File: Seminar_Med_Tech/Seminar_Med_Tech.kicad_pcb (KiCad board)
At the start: 2 copper layers, 96 x 88 mm, 167 parts, among them J1 CONN_02X08, J3 CONN_02X10, J5 CONN_02X10, J6 DB15_F-RA, J7 CONN_02X08, U1 OPA132, U18 ADS1298, U20 ADS1298, U4 LM317T, U5 LM317T, U6 LM337K

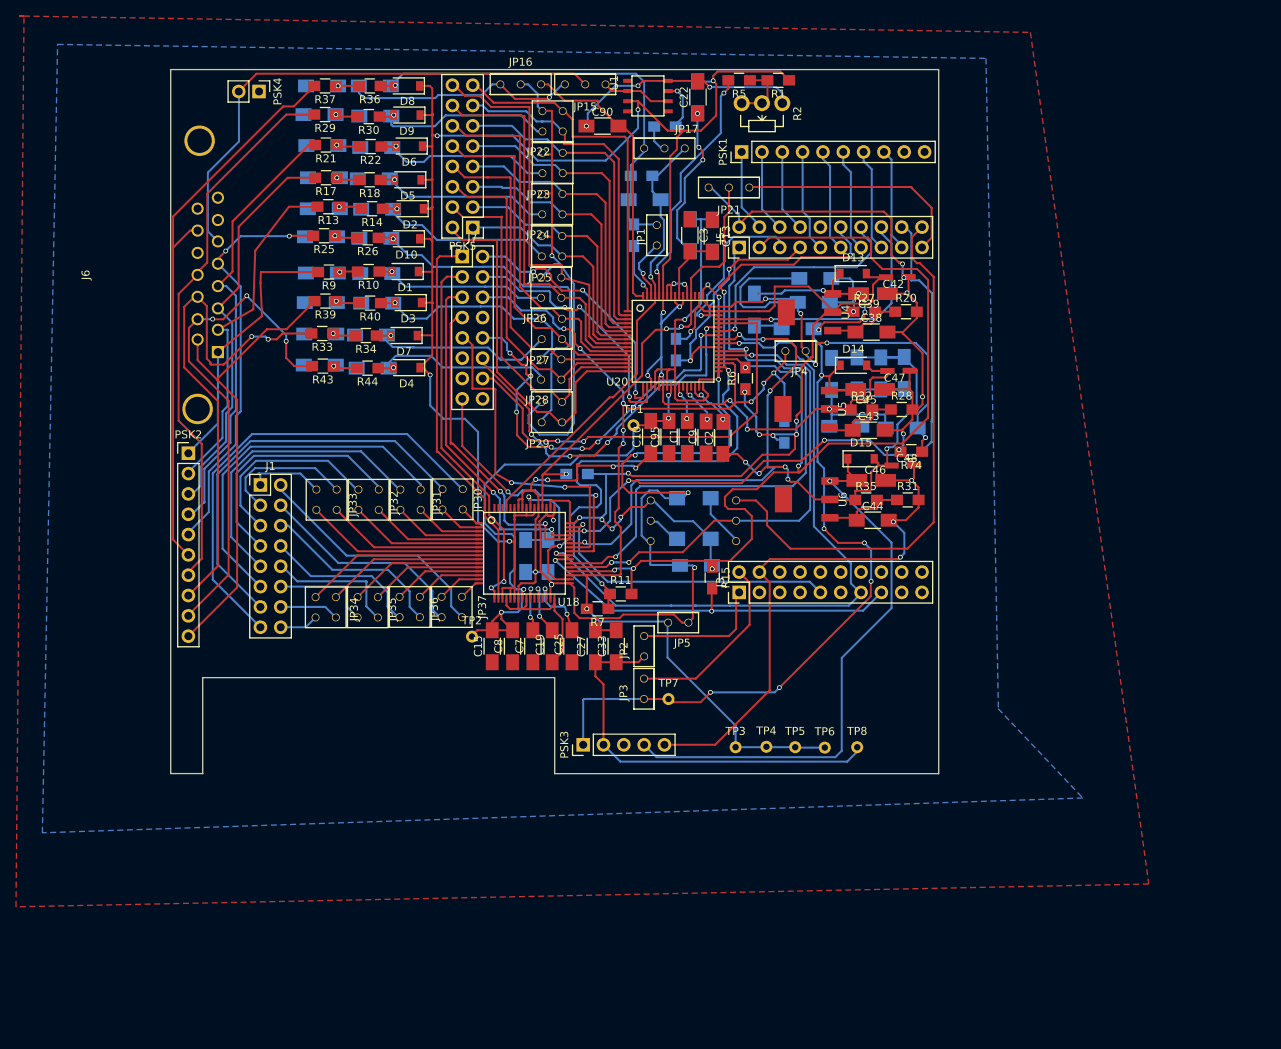
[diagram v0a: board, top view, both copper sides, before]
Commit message: Update
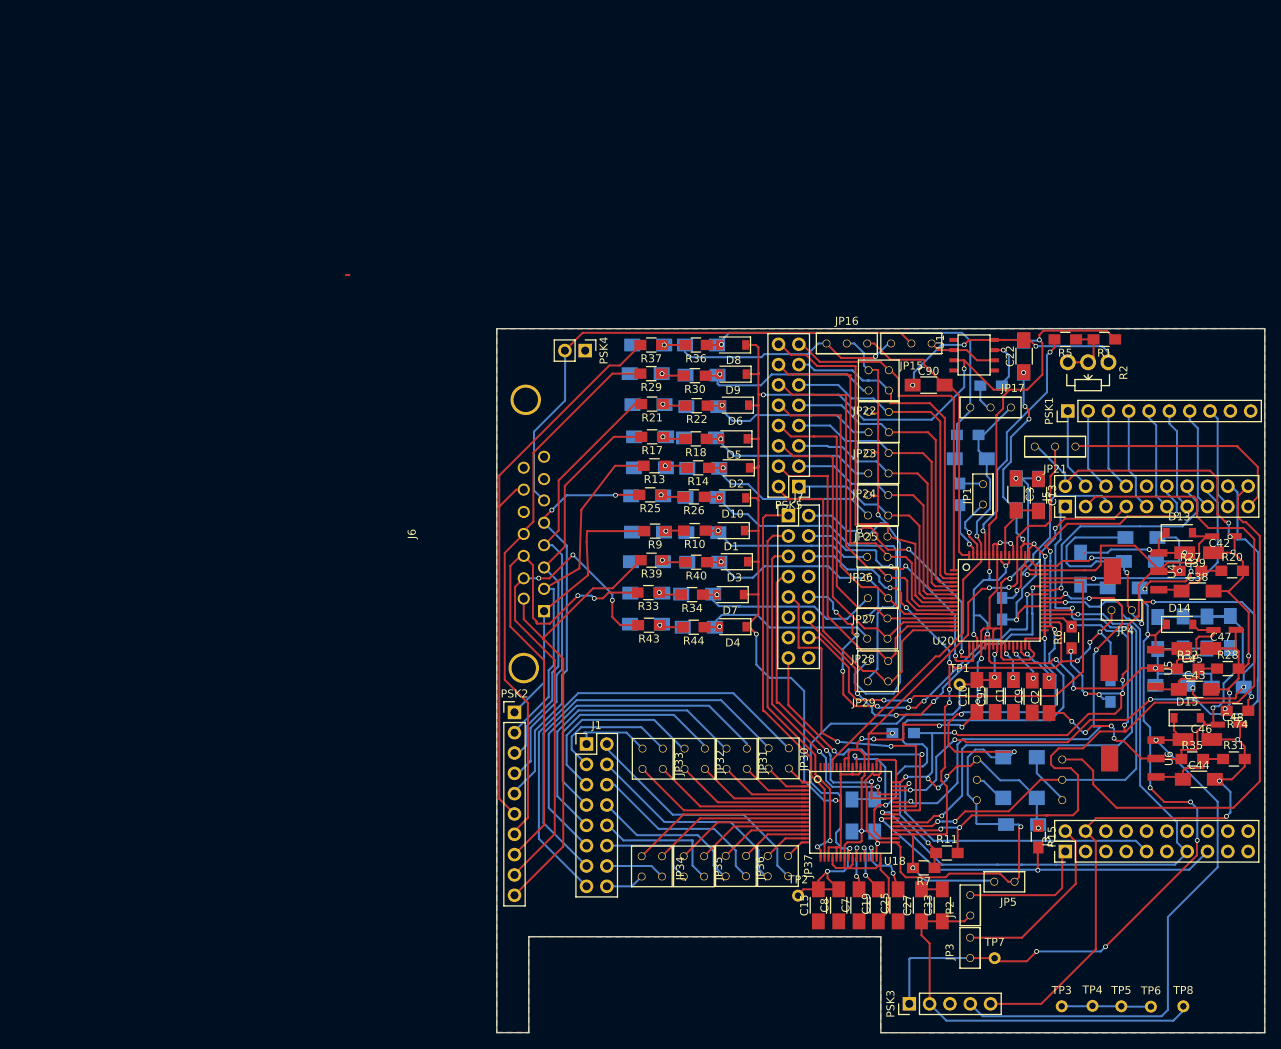
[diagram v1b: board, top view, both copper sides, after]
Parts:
- moved C35 52.2 mm to (139.4, 115.8)
- moved C34 52.1 mm to (136.6, 115.8)
- moved TP6 52.1 mm to (174.0, 139.7)
- moved C42 52.1 mm to (182.5, 81.3)
- moved C48 52.1 mm to (184.2, 104.1)
- moved R32 52.1 mm to (178.6, 97.5)
- moved C15 52.1 mm to (132.4, 127.1)
- moved C22 52.1 mm to (158.1, 58.4)
- moved C23 52.1 mm to (117.4, 92.3)
- moved C24 52.1 mm to (110.8, 91.9)
- moved C27 52.1 mm to (145.3, 127.1)
- moved C33 52.1 mm to (147.9, 127.1)
- moved C74 52.1 mm to (118.0, 84.2)
- moved C80 52.1 mm to (111.3, 72.4)
- moved D2 52.1 mm to (122.1, 72.4)
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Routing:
- net AVSS: track 195.5 -> 214.7 mm, vias 16 -> 20
- net /PWDN: track 111.2 -> 106.8 mm
- net /RESET: track 131.0 -> 132.8 mm
- net AVDD: track 272.1 -> 273.9 mm
- net AGND: track 262.7 -> 264.3 mm, vias 18 -> 20

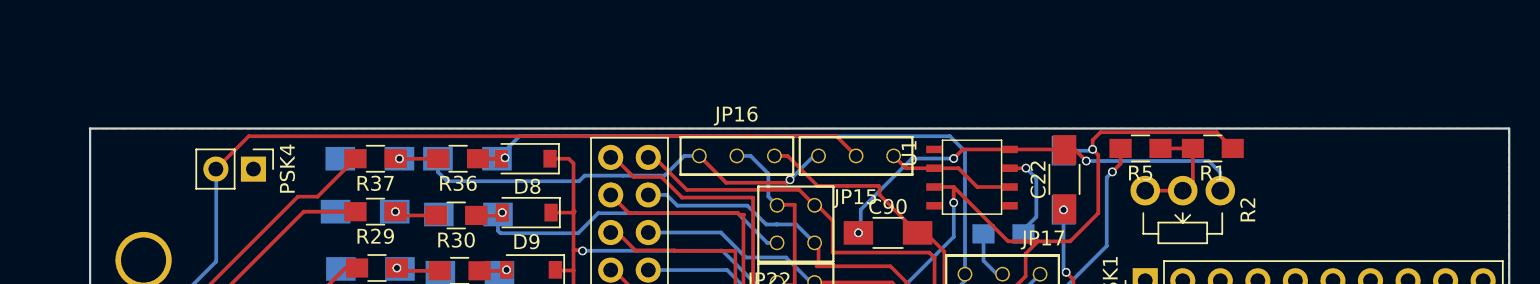
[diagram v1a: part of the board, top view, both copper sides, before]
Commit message: Update
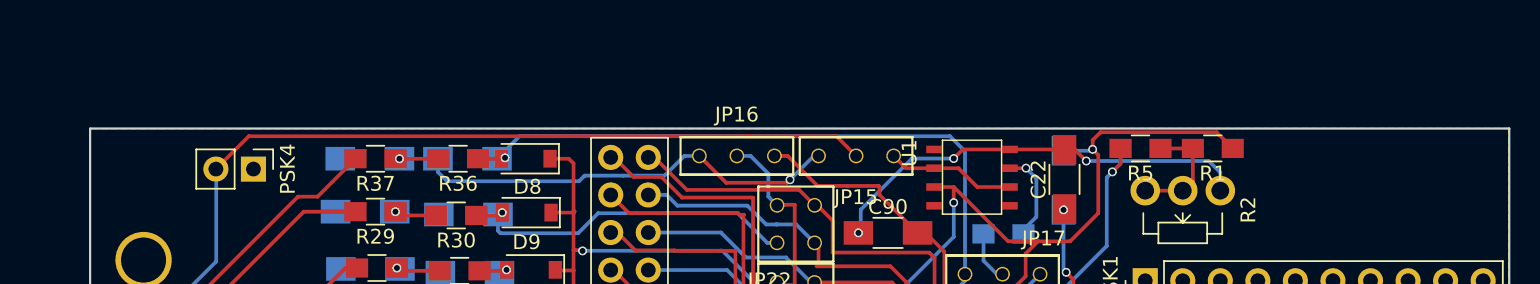
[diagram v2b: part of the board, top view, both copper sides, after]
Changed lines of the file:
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@@
     (links 422)
     (no_connects 0)
-    (area 32.1 15.9 173.700001 127.250001)
+    (area 92.126999 54.903299 188.281301 143.066001)
     (thickness 1.6)
     (drawings 8)
@@
   (gr_line (start 188.202 142.991) (end 140.202 142.991) (angle 90) (layer Edge.Cuts) (width 0.15))
   (gr_line (start 188.202 54.991) (end 188.202 142.991) (angle 90) (layer Edge.Cuts) (width 0.15))
-  (gr_line (start 92.1809 54.9783) (end 188.1809 54.9783) (angle 90) (layer Edge.Cuts) (width 0.15))
+  (gr_line (start 92.2063 54.9783) (end 188.2063 54.9783) (angle 90) (layer Edge.Cuts) (width 0.15))
   (segment (start 165.6715 82.9945) (end 165.7004 82.9656) (width 0.25) (layer F.Cu) (net 0))
   (segment (start 155.7535 94.615) (end 155.7535 95.492) (width 0.25) (layer F.Cu) (net 1))

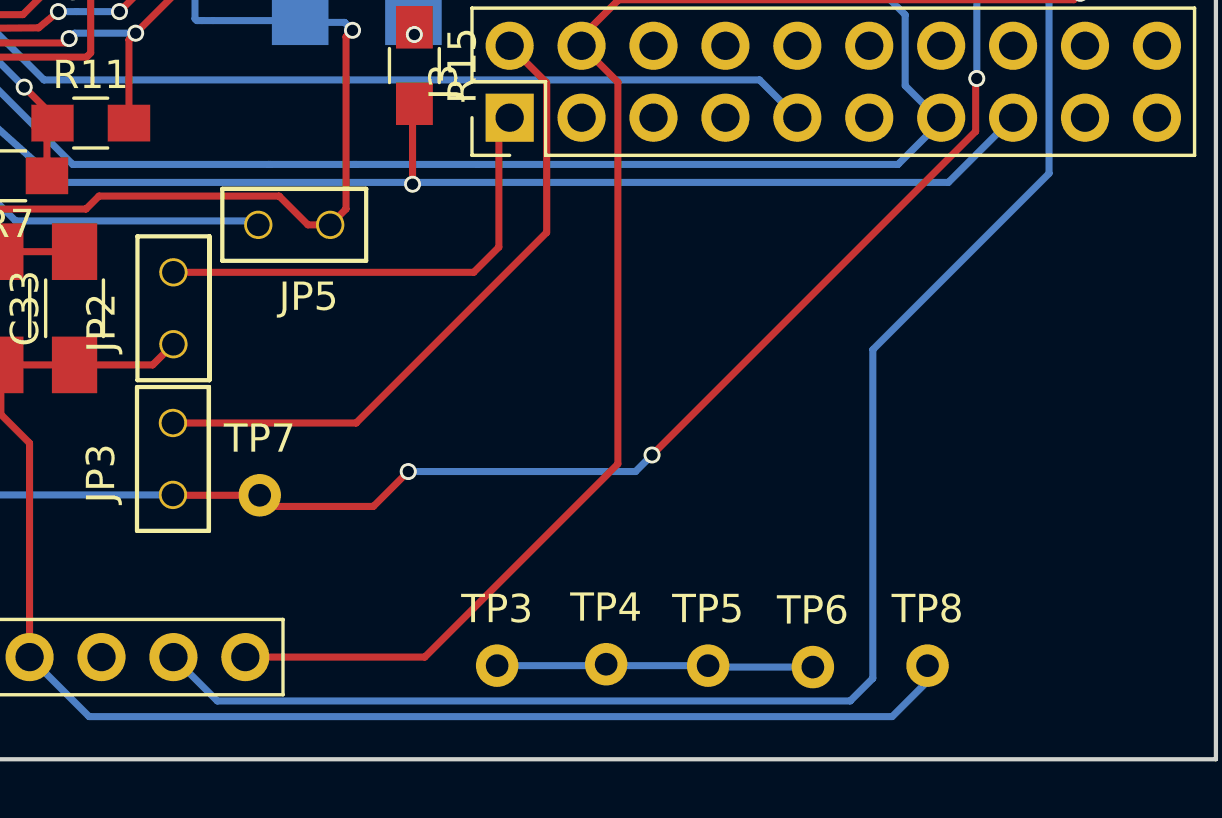
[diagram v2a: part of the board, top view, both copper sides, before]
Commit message: Update
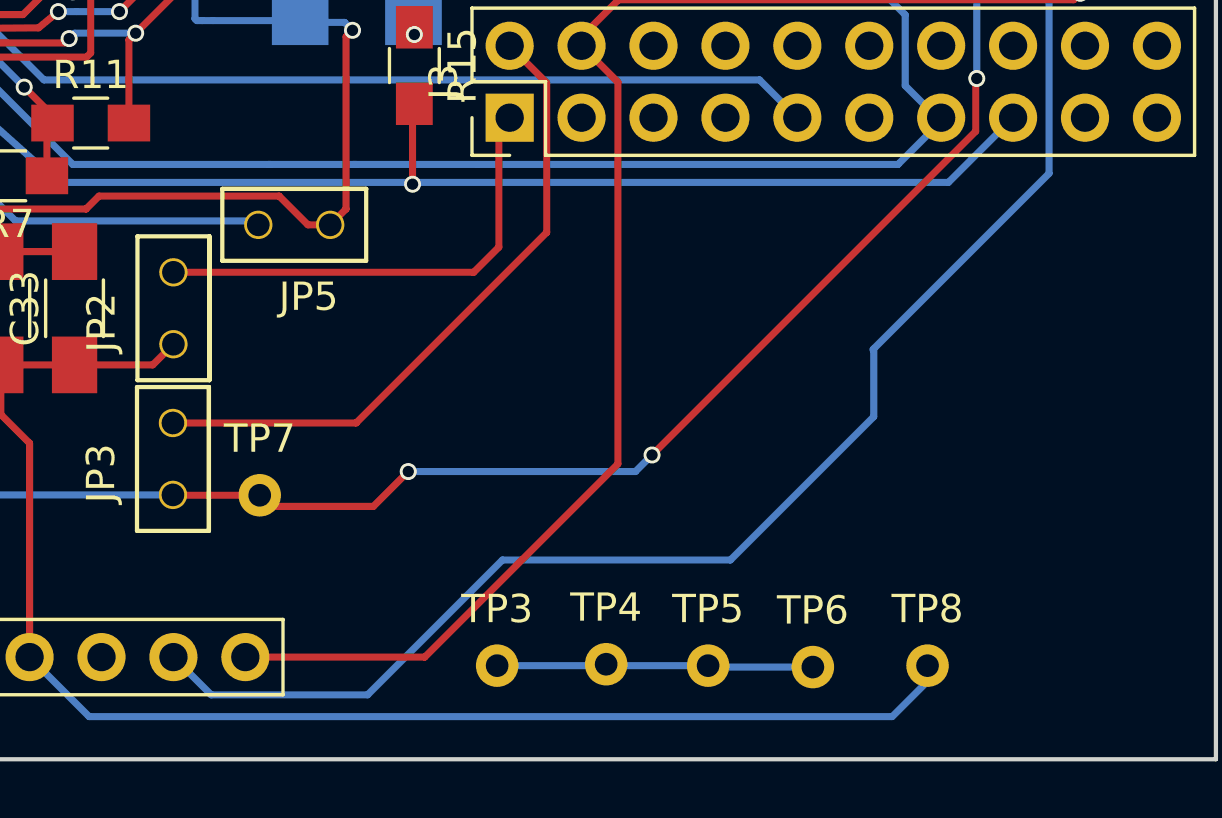
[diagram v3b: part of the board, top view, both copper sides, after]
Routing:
- net -15V_Supply: track 71.7 -> 66.2 mm
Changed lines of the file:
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@@
     (links 422)
     (no_connects 0)
-    (area 92.126999 54.903299 188.281301 143.066001)
+    (area 73.267 48.285 189.841 144.415833)
     (thickness 1.6)
     (drawings 8)
-    (tracks 2422)
+    (tracks 2425)
     (zones 0)
     (modules 167)
@@
     (pad_to_mask_clearance 0.2)
     (aux_axis_origin 0 0)
-    (visible_elements 7FFFFF9F)
+    (visible_elements 7FFFFD9F)
     (pcbplotparams
       (layerselection 0x00030_80000001)
@@
       (padsonsilk false)
       (subtractmaskfromsilk false)
-      (outputformat 1)
+      (outputformat 4)
       (mirror false)
-      (drillshape 1)
+      (drillshape 0)
       (scaleselection 1)
-      (outputdirectory ""))
+      (outputdirectory E:/Seminar/))
   )
   (net 0 "")
@@
   (segment (start 174.604 111.012) (end 177.6555 111.012) (width 0.25) (layer F.Cu) (net 27))
   (segment (start 177.6555 111.012) (end 177.959 111.3155) (width 0.25) (layer F.Cu) (net 27))
+  (segment (start 176.11725 128.49225) (end 176.11725 130.89255) (width 0.25) (layer B.Cu) (net 28))
+  (segment (start 158.242 140.716) (end 152.7175 140.716) (width 0.25) (layer B.Cu) (net 28))
+  (segment (start 163.0045 135.9535) (end 158.242 140.716) (width 0.25) (layer B.Cu) (net 28))
+  (segment (start 171.0563 135.9535) (end 163.0045 135.9535) (width 0.25) (layer B.Cu) (net 28))
+  (segment (start 176.11725 130.89255) (end 171.0563 135.9535) (width 0.25) (layer B.Cu) (net 28))
   (via (at 174.604 106.412) (size 0.6) (drill 0.4) (layers F.Cu B.Cu) (net 28))
   (segment (start 177.9015 106.412) (end 174.604 106.412) (width 0.25) (layer F.Cu) (net 28))
-  (segment (start 152.9334 140.9319) (end 151.384 139.3825) (width 0.25) (layer B.Cu) (net 28))
-  (segment (start 175.286898 140.9319) (end 152.9334 140.9319) (width 0.25) (layer B.Cu) (net 28))
-  (segment (start 176.0855 140.133298) (end 175.286898 140.9319) (width 0.25) (layer B.Cu) (net 28))
-  (segment (start 176.0855 128.524) (end 176.0855 140.133298) (width 0.25) (layer B.Cu) (net 28))
-  (segment (start 182.3085 122.301) (end 176.0855 128.524) (width 0.25) (layer B.Cu) (net 28))
+  (segment (start 152.7175 140.716) (end 151.384 139.3825) (width 0.25) (layer B.Cu) (net 28))
+  (segment (start 182.3085 122.301) (end 176.11725 128.49225) (width 0.25) (layer B.Cu) (net 28))
+  (segment (start 176.11725 128.49225) (end 176.0855 128.524) (width 0.25) (layer B.Cu) (net 28))
   (segment (start 182.3085 114.1165) (end 182.3085 122.301) (width 0.25) (layer B.Cu) (net 28))
   (segment (start 174.604 106.412) (end 182.3085 114.1165) (width 0.25) (layer B.Cu) (net 28))
